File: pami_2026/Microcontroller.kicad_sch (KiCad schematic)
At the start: 1 part, among them U1 ESP32-WROOM-E

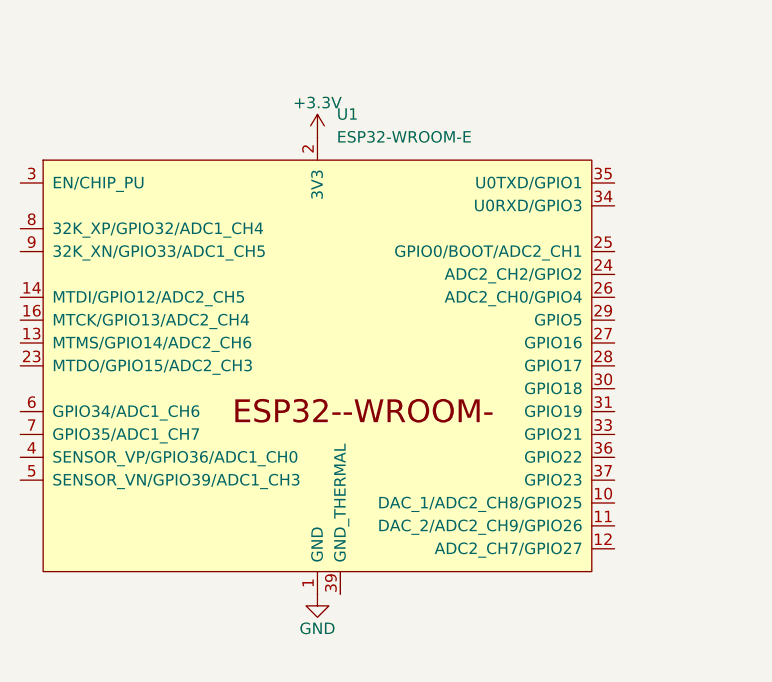
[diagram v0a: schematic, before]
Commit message: WIP actuators
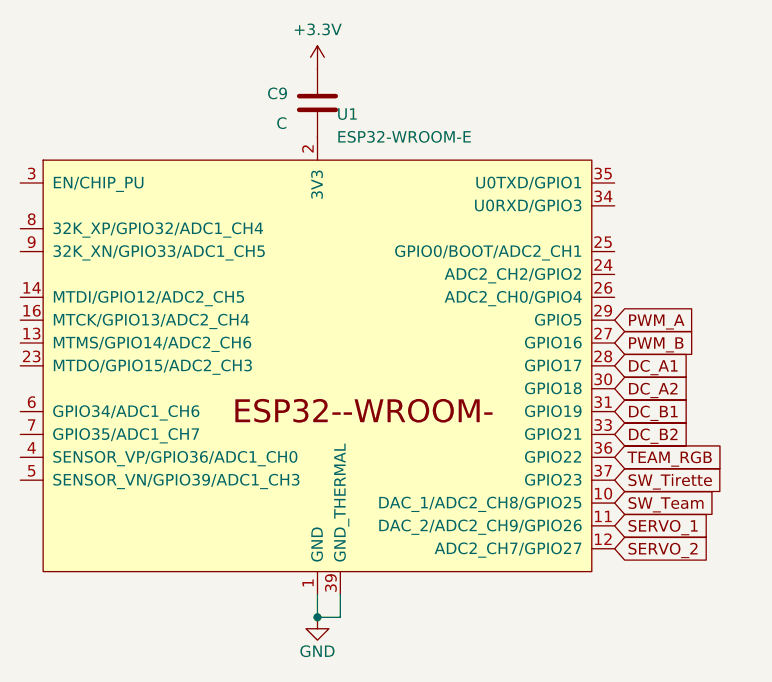
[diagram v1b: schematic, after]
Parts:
- added C9: C, symbol Device:C
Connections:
- net +3.3V: now also C9.1; no longer U1.2 (3V3)
- net GND: now also U1.39 (GND_THERMAL)
- net SW_Team: now reaches U1.10 (DAC_1/ADC2_CH8/GPIO25)
- net SERVO_1: now reaches U1.11 (DAC_2/ADC2_CH9/GPIO26)
- net SERVO_2: now reaches U1.12 (ADC2_CH7/GPIO27)
- net PWM_B: now reaches U1.27 (GPIO16)
- net DC_A1: now reaches U1.28 (GPIO17)
- net PWM_A: now reaches U1.29 (GPIO5)
- net DC_A2: now reaches U1.30 (GPIO18)
- net DC_B1: now reaches U1.31 (GPIO19)
- net DC_B2: now reaches U1.33 (GPIO21)
- net TEAM_RGB: now reaches U1.36 (GPIO22)
- net SW_Tirette: now reaches U1.37 (GPIO23)
- new net: C9.2, U1.2 (3V3)
